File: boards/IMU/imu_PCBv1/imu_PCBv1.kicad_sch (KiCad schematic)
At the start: 30 parts, among them J1 USB_B_Mini, J2 SWD_Header, J4 Micro_SD_Card_Det1, J5 UART, J6 CAN_Bus, U1 ISM330DLCTR, U2 STM32F103RBT6, U3 SN65HVD230, U4 AP2112K-3.3, Y1 8MHz

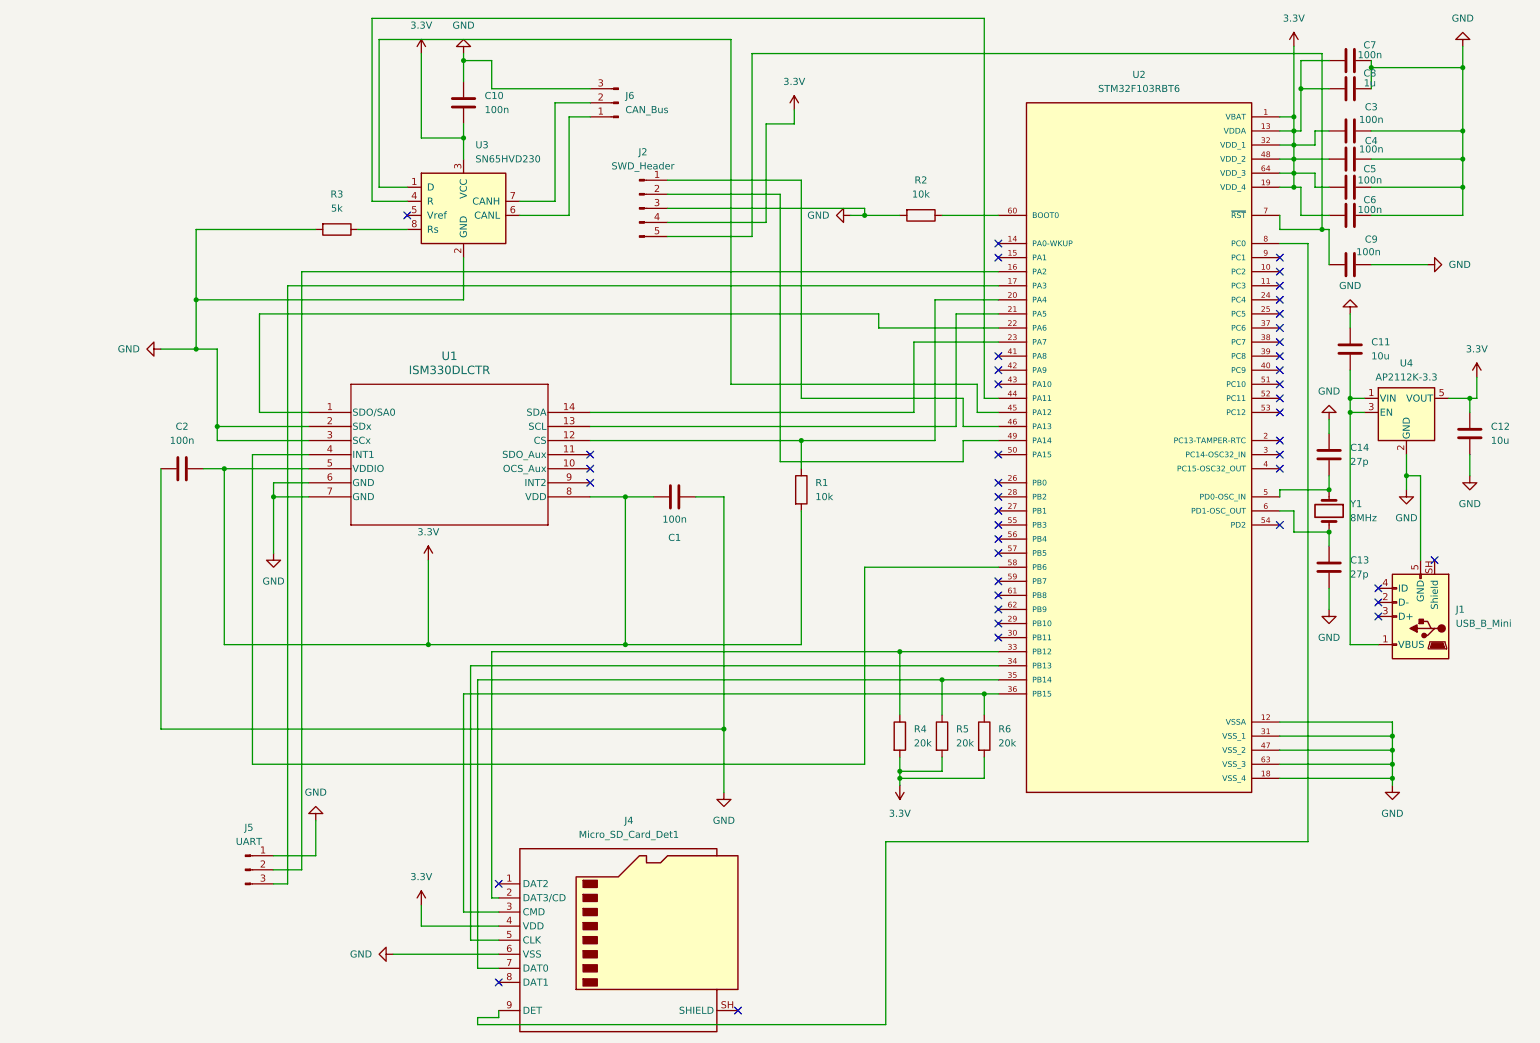
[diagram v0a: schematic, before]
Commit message: Organized first draft of schematic
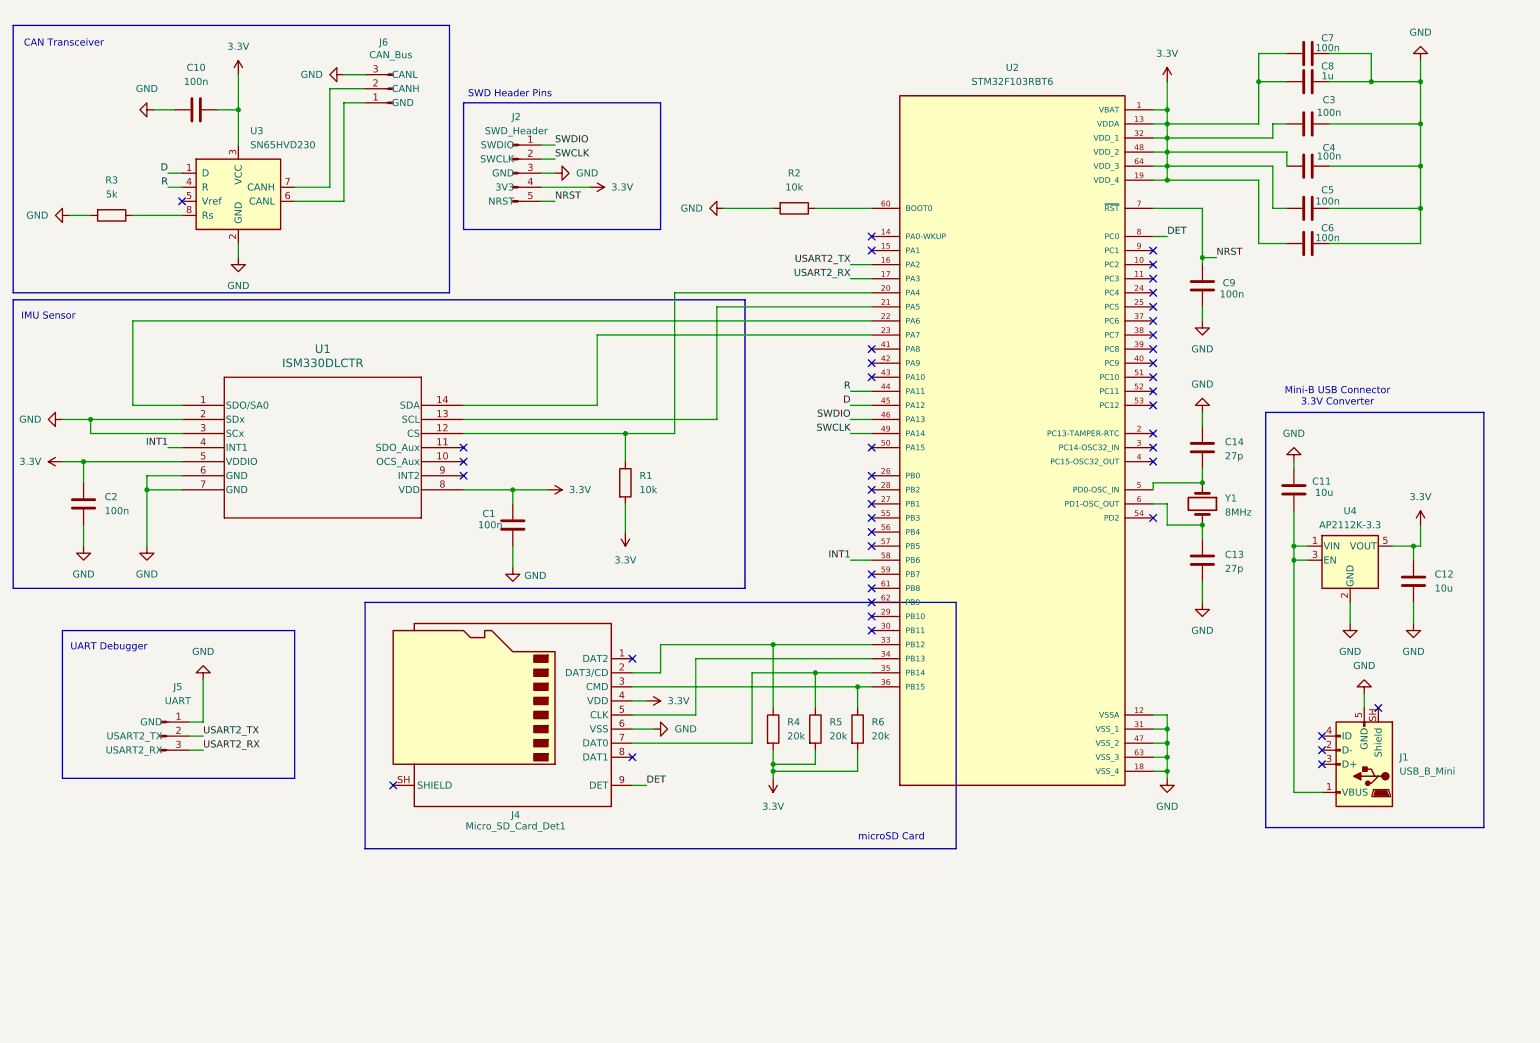
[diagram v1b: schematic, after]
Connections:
- net 3.3V: now also C2.2; no longer C2.1
- net GND: now also C2.1; no longer C2.2
- net SWDIO: now reaches J2.1 (SWDIO), U2.46 (PA13)
- net SWCLK: now reaches J2.2 (SWCLK), U2.49 (PA14)
- net NRST: now reaches C9.2, J2.5 (NRST), U2.7 (~{RST})
- net DET: now reaches J4.9 (DET), U2.8 (PC0)
- net USART2_TX: now reaches J5.2 (USART2_TX), U2.16 (PA2)
- net USART2_RX: now reaches J5.3 (USART2_RX), U2.17 (PA3)
- net R: now reaches U2.44 (PA11), U3.4 (R)
- net D: now reaches U2.45 (PA12), U3.1 (D)
- net INT1: now reaches U1.4 (INT1), U2.58 (PB6)
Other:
- note added: "CAN Transceiver"
- note added: "IMU Sensor"
- note added: "Mini-B USB Connector 3.3V Converter"
- note added: "SWD Header Pins"
- note added: "UART Debugger"
- note added: "microSD Card"
- moved on the sheet: C1, C10, C11, C12, C13, C14, C2, C3, C4, C5, C6, C7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
